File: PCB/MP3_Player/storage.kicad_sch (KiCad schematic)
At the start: 8 parts, among them J6 Micro_SD_Card

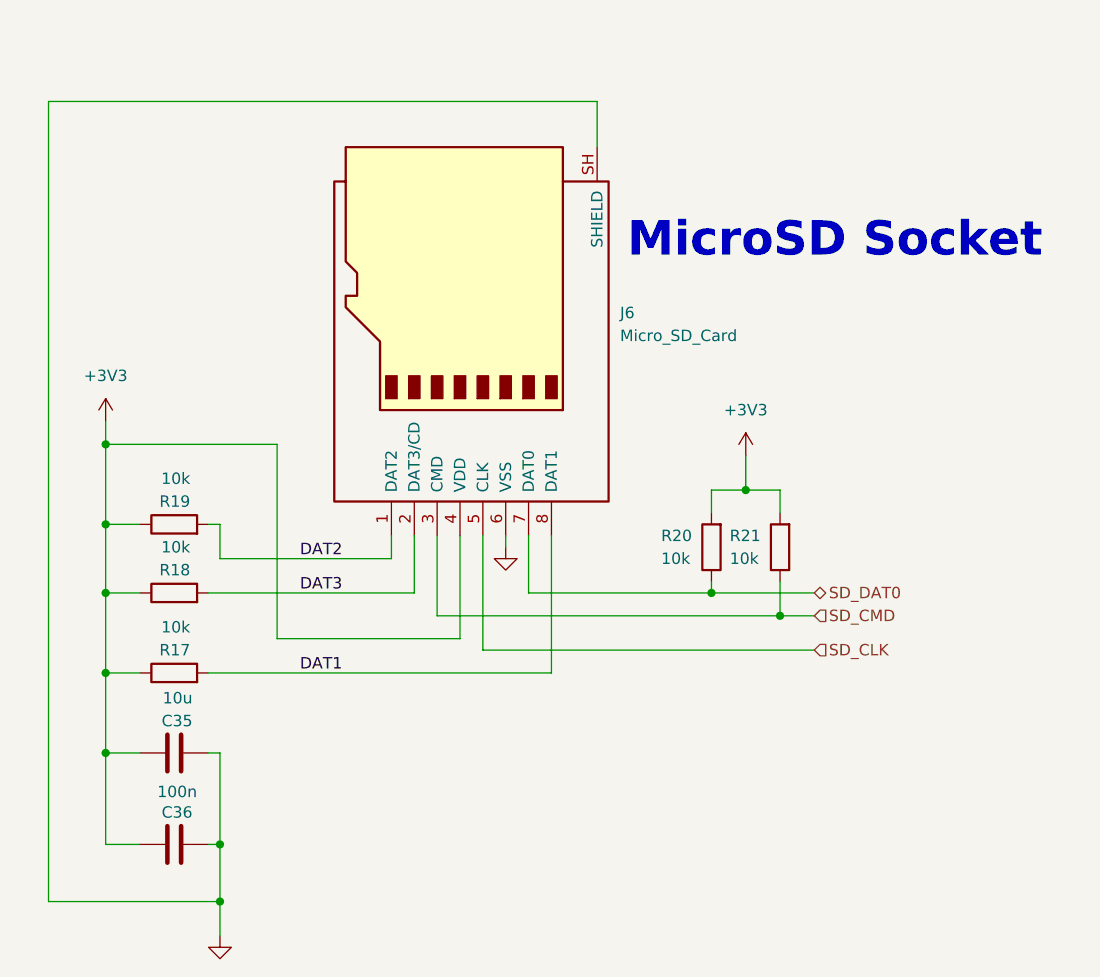
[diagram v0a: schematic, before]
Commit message: Minor Schematic Changes
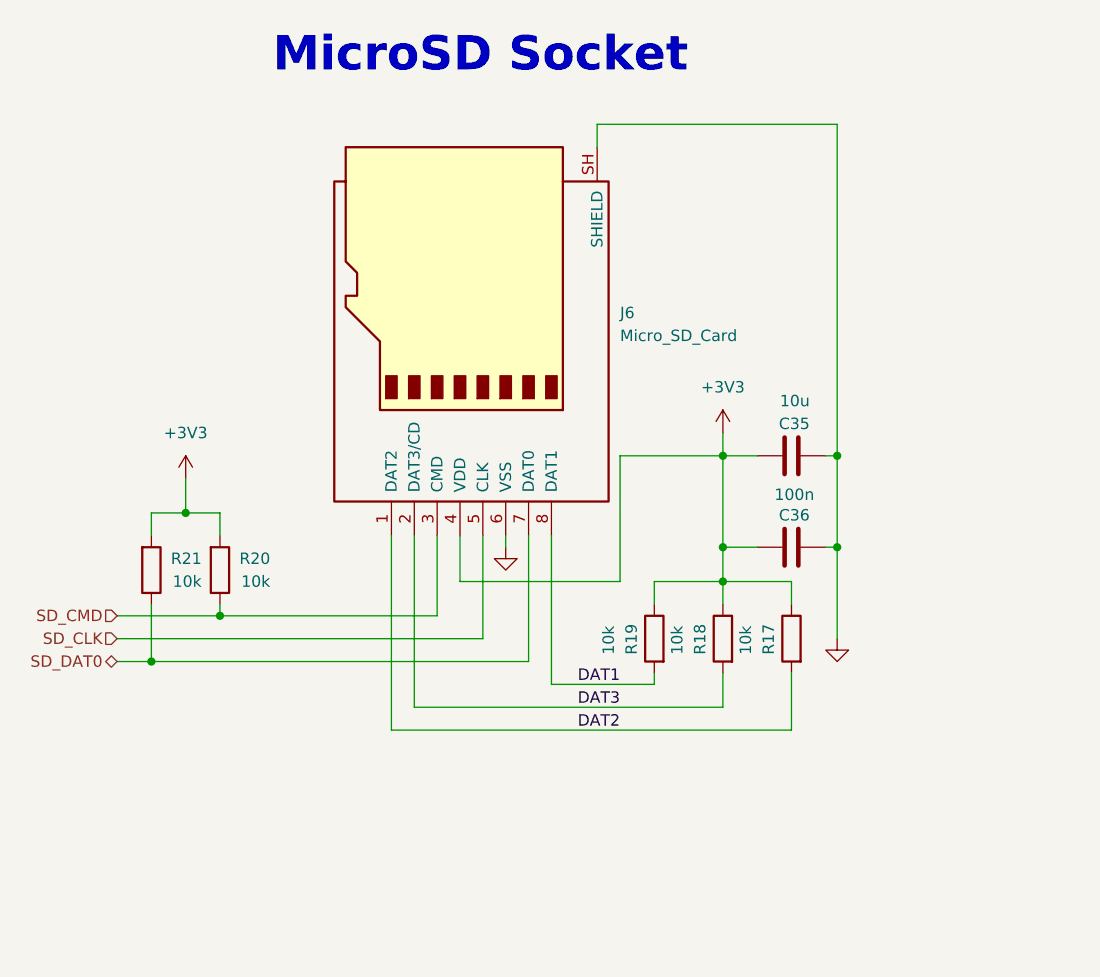
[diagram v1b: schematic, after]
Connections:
- net DAT1: now also R19.2; no longer R17.2
- net DAT2: now also R17.2; no longer R19.2
- net SD_CMD: now also R20.1; no longer R21.1
- net SD_DAT0: now also R21.1; no longer R20.1
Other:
- moved on the sheet: C35, C36
